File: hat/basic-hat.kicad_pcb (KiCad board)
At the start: 4 copper layers, 65 x 56.5 mm, 45 parts, among them IC1 LM2676S-5.0, IC2 DMMT5401-7-F, J1 Conn_Coaxial, J2 nfc, J3 52840 tx pri rx, J4 52840 rx rpi tx, J5 Raspberry_Pi_2_3, J6 Conn_ARM_JTAG_SWD_10, J7 Screw_Terminal_01x02, J8 Screw_Terminal_01x01, Q1 DMG2305UX-7, U1 nrf52840, Y1 32mhzCrystal

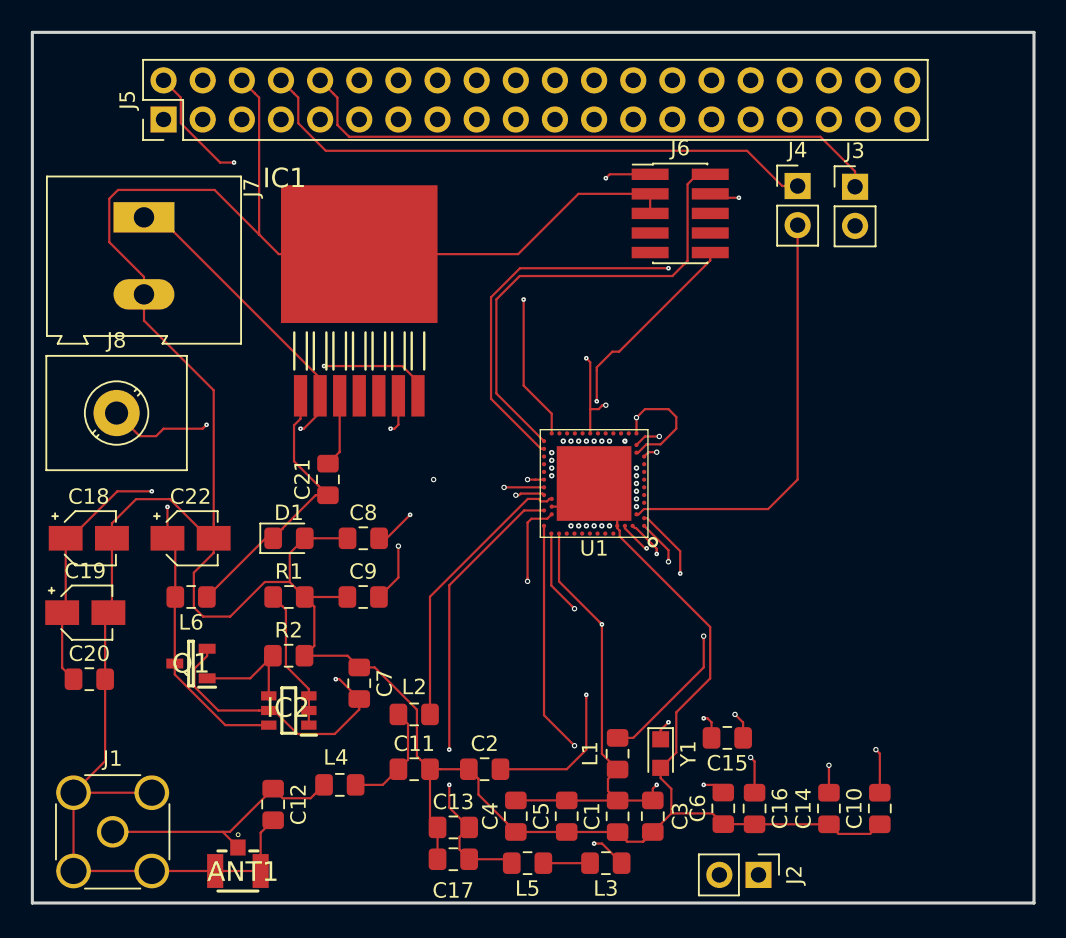
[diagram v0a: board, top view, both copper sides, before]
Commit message: optimized layout
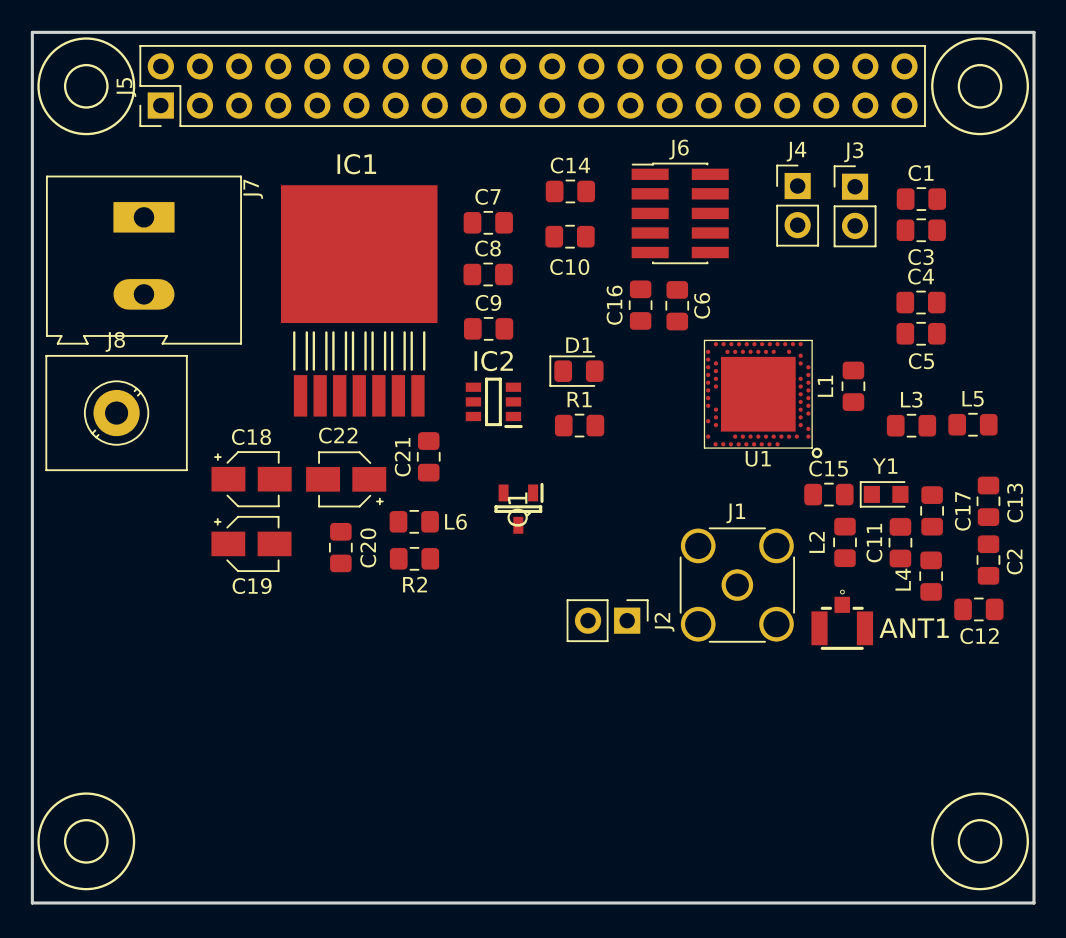
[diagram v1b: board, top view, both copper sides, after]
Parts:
- moved C12 47.5 mm to (101.4, 57.5), turned to 0 degrees
- moved C1 44.6 mm to (97.7, 30.8), turned to 0 degrees
- moved J1 43.6 mm to (85.8, 55.9)
- moved C14 43.4 mm to (74.9, 30.3), turned to 0 degrees
- moved C4 42.5 mm to (97.7, 37.5), turned to 0 degrees
- moved ANT1 42.3 mm to (92.6, 58.7)
- moved C10 42.2 mm to (74.9, 33.3), turned to 0 degrees
- moved C3 41.8 mm to (97.7, 32.8), turned to 0 degrees
- moved L4 40.7 mm to (98.3, 55.3), turned to 270 degrees
- moved C13 40.7 mm to (102.0, 50.4), turned to 90 degrees
- moved L5 40.6 mm to (101.0, 45.5), turned to 0 degrees
- moved C5 38.8 mm to (97.7, 39.6), turned to 0 degrees
- moved C17 38.4 mm to (98.4, 51.1), turned to 90 degrees
- moved C2 35.4 mm to (102.0, 54.2), turned to 90 degrees
- moved C11 34.8 mm to (96.3, 53.1), turned to 90 degrees
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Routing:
- net Ground (VSS_PA): track 237.4 -> 0.00 mm
- net VDDH: track 99.7 -> 0.00 mm, vias 5 -> 0
- net VDD(A22): track 91.4 -> 0.00 mm, vias 9 -> 0
- net 1.3vsup_decup(dec4): track 50.3 -> 0.00 mm, vias 3 -> 0
- net +12V: track 47.4 -> 0.00 mm, vias 2 -> 0
- net P0.09: track 40.6 -> 0.00 mm, vias 1 -> 0
- net Net-(J3-Pad1): track 39.2 -> 0.00 mm
- net P0.10: track 38.4 -> 0.00 mm, vias 1 -> 0
- net Net-(C22-Pad1): track 37.6 -> 0.00 mm, vias 2 -> 0
- net Net-(J4-Pad1): track 37.3 -> 0.00 mm
- net 1.3vsup_decup(flash)(dec5): track 35.6 -> 0.00 mm, vias 2 -> 0
- net SWDCLK: track 34.6 -> 0.00 mm, vias 2 -> 0
- net psu_decup(dec3): track 31.9 -> 0.00 mm, vias 2 -> 0
- net P0.01: track 30.8 -> 0.00 mm, vias 1 -> 0
- net SWDIO: track 30.6 -> 0.00 mm
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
